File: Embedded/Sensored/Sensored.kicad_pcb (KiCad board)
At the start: 2 copper layers, 9 x 9.5 mm, 13 parts, among them U1 ICM-20948, U3 BME280

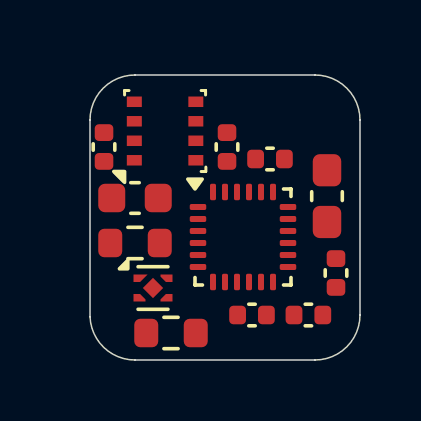
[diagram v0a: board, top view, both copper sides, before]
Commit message: Added Castellated Pins & Removed Micro SD Card
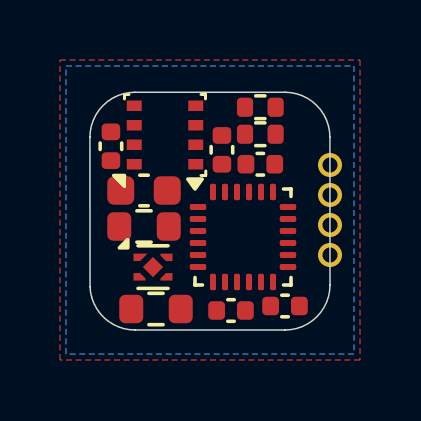
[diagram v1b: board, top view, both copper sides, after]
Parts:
- removed C10: 22uF, Capacitor_SMD:C_0603_1608Metric_Pad1.08x0.95mm_HandSolder
- removed C12: 0.1uF, Capacitor_SMD:C_0402_1005Metric
- added J1: Casselation, Simple_Connector:1mm_4P, F.Cu at (146.0, 109.5)
- added R1: 10K, Resistor_SMD:R_0402_1005Metric, F.Cu at (143.7, 105.5)
- added R2: 10K, Resistor_SMD:R_0402_1005Metric, F.Cu at (143.7, 104.6)
- moved C9 0.94 mm to (140.2, 111.3)
- moved C3 0.84 mm to (144.5, 111.2)
- moved C4 0.72 mm to (142.7, 111.3)
- moved U4 0.70 mm to (140.1, 109.9)
- moved C11 0.63 mm to (139.8, 108.5)
- moved C13 0.39 mm to (139.8, 107.3)
- moved C1 0.37 mm to (143.7, 106.5)
- moved C6 0.23 mm to (138.7, 105.9)
- moved C8 0.19 mm to (142.4, 106.0)
- moved U3 0.13 mm to (140.5, 105.5)
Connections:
- C9 pad 1: Vin -> +3V3
- U4 pad 3: Vin -> +3V3
- U4 pad 4: Vin -> +3V3
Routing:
- added copper zone on F.Cu, net +3V3
- added copper zone on B.Cu, net GND
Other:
- board size 9 x 9.5 mm -> 8 x 7.9 mm
